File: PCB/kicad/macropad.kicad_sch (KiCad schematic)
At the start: 94 parts, among them J1 OLED_128x32, J2 4P4C, SW1 RESET_Push, SW2 RotaryEncoder_Switch, SW3 RotaryEncoder_Switch, SW4 RotaryEncoder_Switch, SW5 Soft_Push, SW6 Soft_Push, SW7 Soft_Push, U1 5-Way Nav, U2 ON/OFF

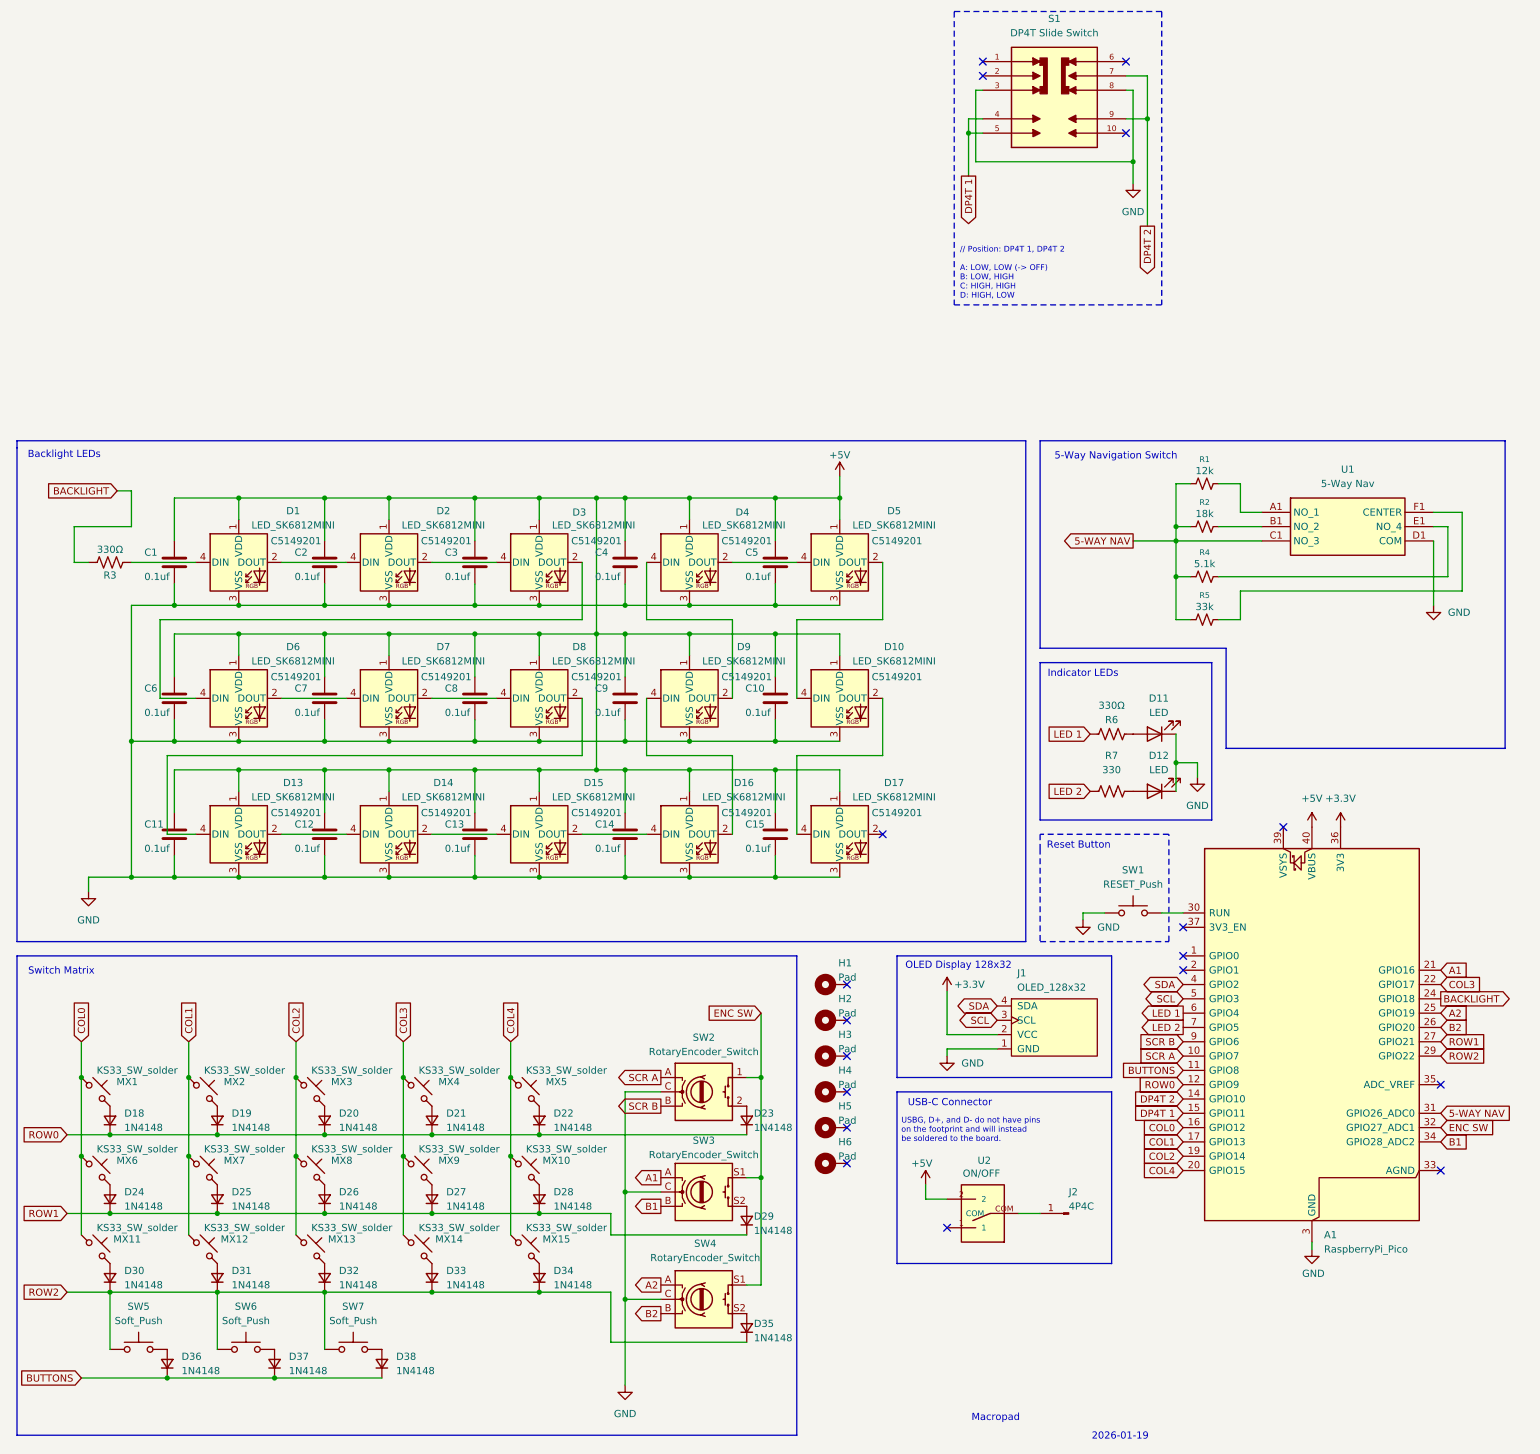
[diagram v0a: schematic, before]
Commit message: Routed PCB v2
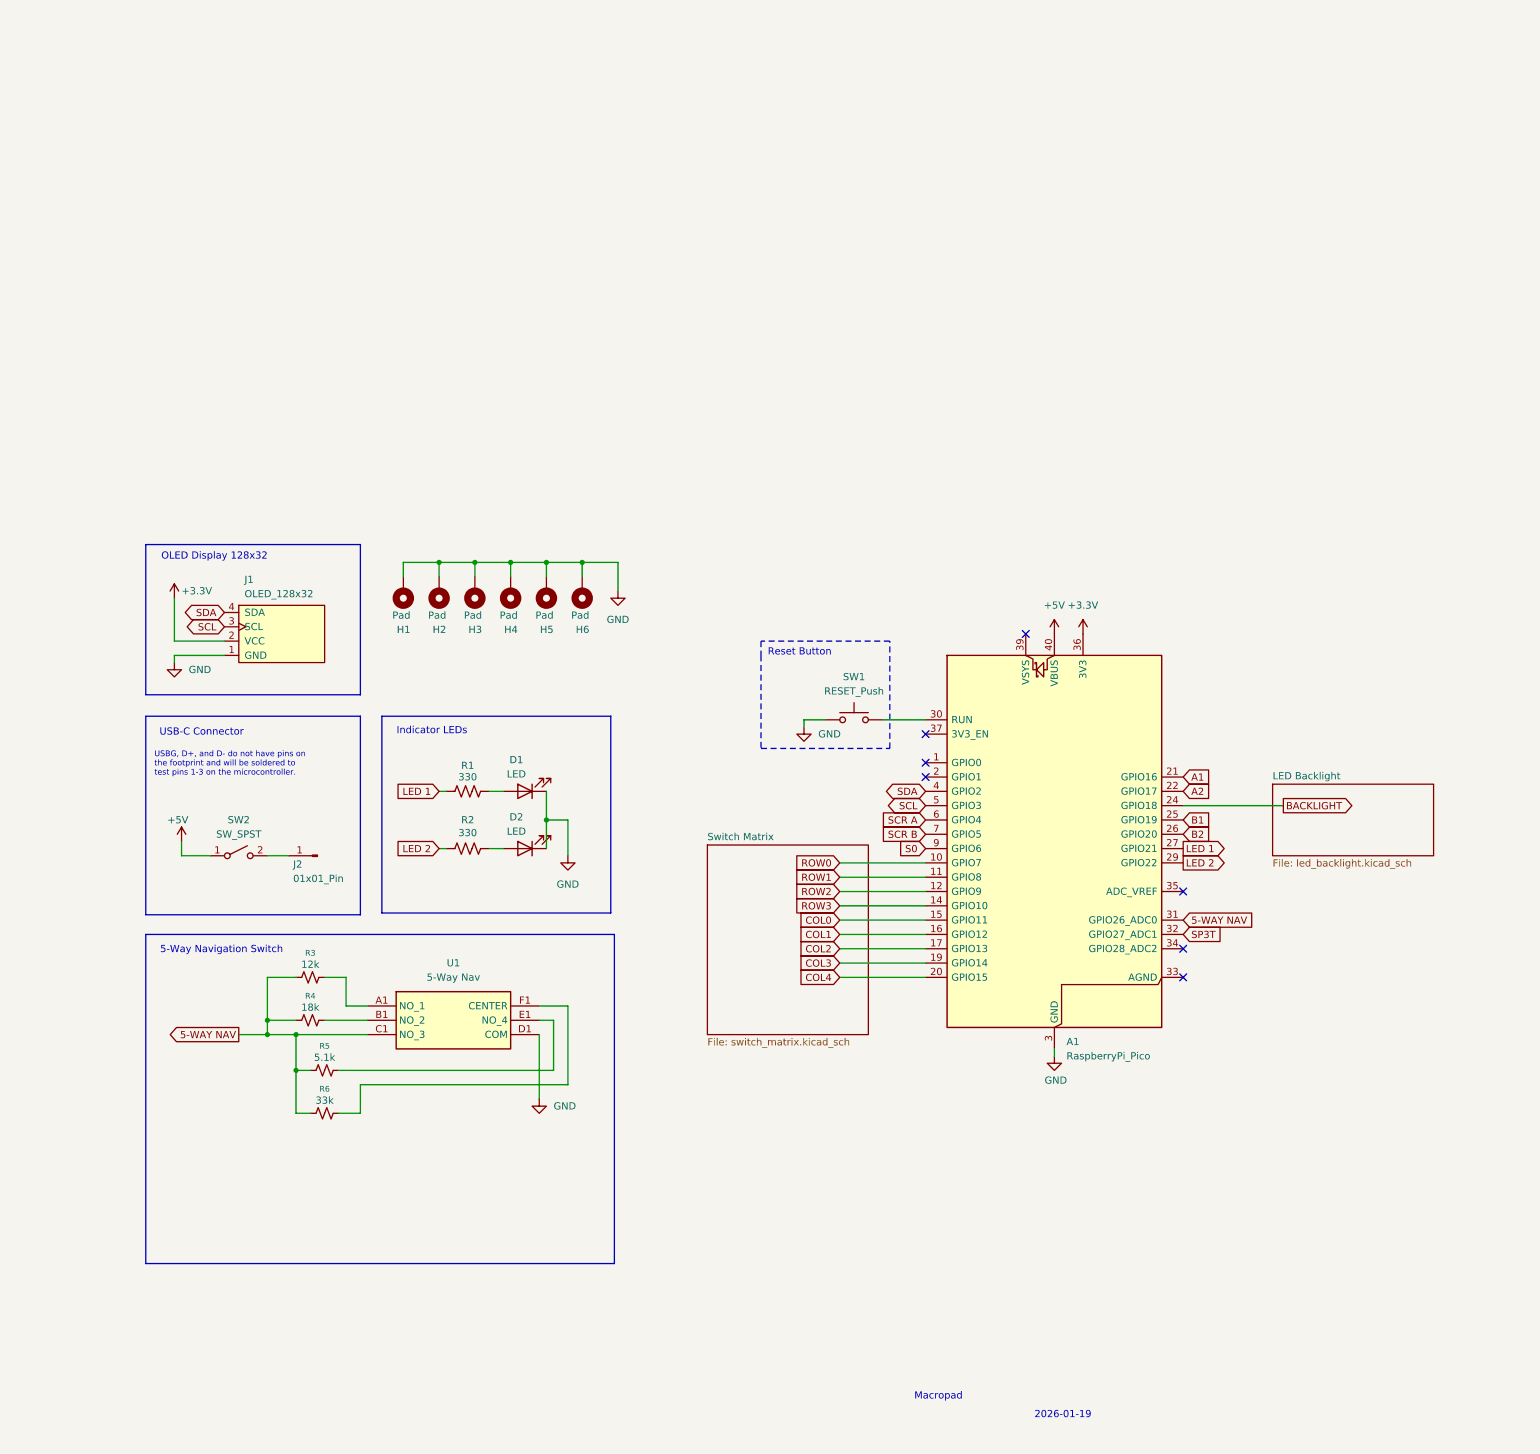
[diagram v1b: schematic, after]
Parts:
- removed C1, C10, C11, C12, C13, C14, C15, C2, C3, C4, C5, C6, C7, C8, C9: 0.1uf, Capacitor_SMD:C_1206_3216Metric, symbol Device:C
- removed D1, D10, D13, D14, D15, D16, D17, D2, D3, D4, D5, D6, D7, D8, D9: LED_SK6812MINI, macropad_components:LED_SK6812MINI, symbol ScottoKeebs:LED_SK6812MINI
- removed D18, D19, D20, D21, D22, D23, D24, D25, D26, D27, D28, D29, D30, D31, D32, D33, D34, D35, D36, D37, D38: 1N4148, macropad_components:Diode_DO-35, symbol Device:D_Small
- removed MX1, MX10, MX11, MX12, MX13, MX14, MX15, MX2, MX3, MX4, MX5, MX6, MX7, MX8, MX9: KS33_SW_solder, macropad_components:SW_KS33_1u, symbol Switch:SW_Push_45deg
- removed R3: 330Ω, Resistor_THT:R_Axial_DIN0207_L6.3mm_D2.5mm_P10.16mm_Horizontal, symbol Device:R_US
- removed S1: DP4T Slide Switch, Connector_PinHeader_2.54mm:PinHeader_2x06_P2.54mm_Vertical, symbol SLW-18115106-5A-RA-S-D:SLW-18115106-5A-RA-S-D
- removed SW2: RotaryEncoder_Switch, macropad_components:CKW12, symbol Device:RotaryEncoder_Switch
- removed SW3, SW4: RotaryEncoder_Switch, Rotary_Encoder:RotaryEncoder_Alps_EC11E-Switch_Vertical_H20mm, symbol Device:RotaryEncoder_Switch
- removed SW5, SW6, SW7: Soft_Push, Button_Switch_THT:SW_PUSH_6mm, symbol Switch:SW_Push
- removed U2: ON/OFF, macropad_components:SK12D07VG4, symbol SK12D07VG4:SK12D07VG4
- added SW2: SW_SPST, Button_Switch_SMD:SW_DIP_SPSTx01_Slide_6.7x4.1mm_W6.73mm_P2.54mm_LowProfile_JPin, symbol Switch:SW_SPST
- J1: footprint Connector_Wire:SolderWire-0.25sqmm_1x04_P4.2mm_D0.65mm_OD1.7mm -> Connector_PinHeader_2.54mm:PinHeader_1x04_P2.54mm_Vertical
- J2: value 4P4C -> 01x01_Pin
- R1: renamed from R6; value 330Ω -> 330
- renumbered D11 to D1, D12 to D2, R7 to R2, R1 to R3, R2 to R4, R4 to R5, R5 to R6
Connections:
- net BUTTONS is gone; now on net ROW1: A1.11 (GPIO8)
- net DP4T 1 is gone; now on net COL0: A1.15 (GPIO11)
- net +5V: now also SW2.1 (A)
- net A2: now also A1.22 (GPIO17); no longer A1.25 (GPIO19)
- net B1: now also A1.25 (GPIO19); no longer A1.34 (GPIO28_ADC2)
- net COL0: no longer A1.16 (GPIO12)
- net COL1: now also A1.16 (GPIO12); no longer A1.17 (GPIO13)
- net COL2: now also A1.17 (GPIO13); no longer A1.19 (GPIO14)
- net COL3: now also A1.19 (GPIO14); no longer A1.22 (GPIO17)
- net GND: now also H1.1, H2.1, H3.1, H4.1, H5.1, H6.1
- net LED 1: now also A1.27 (GPIO21); no longer A1.6 (GPIO4)
- net LED 2: now also A1.29 (GPIO22); no longer A1.7 (GPIO5)
- net ROW0: now also A1.10 (GPIO7); no longer A1.12 (GPIO9)
- net ROW1: no longer A1.27 (GPIO21)
- net ROW2: now also A1.12 (GPIO9); no longer A1.29 (GPIO22)
- net SCR A: now also A1.6 (GPIO4); no longer A1.10 (GPIO7)
- net SCR B: now also A1.7 (GPIO5); no longer A1.9 (GPIO6)
- net at J2.1 (Pin_1): now also SW2.2 (B)
- net DP4T 2 renamed ROW3
- net ENC SW renamed SP3T
- new net S0: A1.9 (GPIO6)
- no-connect marks 18 -> 7
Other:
- added sheet LED Backlight (led_backlight.kicad_sch)
- added sheet Switch Matrix (switch_matrix.kicad_sch)
- note added: "USBG, D+, and D- do not have pins on the footprint and will be soldered to test pins 1-3 on the microcontroller."
- note removed: "// Position: DP4T 1, DP4T 2 A: LOW, LOW (-> OFF) B: LOW, HIGH C: HIGH, HIGH D: HIGH, LOW"
- note removed: "Backlight LEDs"
- note removed: "Switch Matrix"
- note removed: "USBG, D+, and D- do not have pins on the footprint and will instead be soldered to the board."
- moved on the sheet: A1, D1, D2, H1, H2, H3, H4, H5, H6, J1, J2, R1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
